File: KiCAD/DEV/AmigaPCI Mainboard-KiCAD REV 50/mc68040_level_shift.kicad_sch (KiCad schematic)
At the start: 28 parts, among them U801 74LVC1G17, U802 SN74LVC16T245DLR, U803 SN74LVC16T245DLR, U804 SN74LVC16T245DLR, U805 SN74LVC16T245DLR, U806 74LVC245, U807 74LVC245, U808 74LVC245, U809 74LVC245, U810 SN74LVC16T245DLR

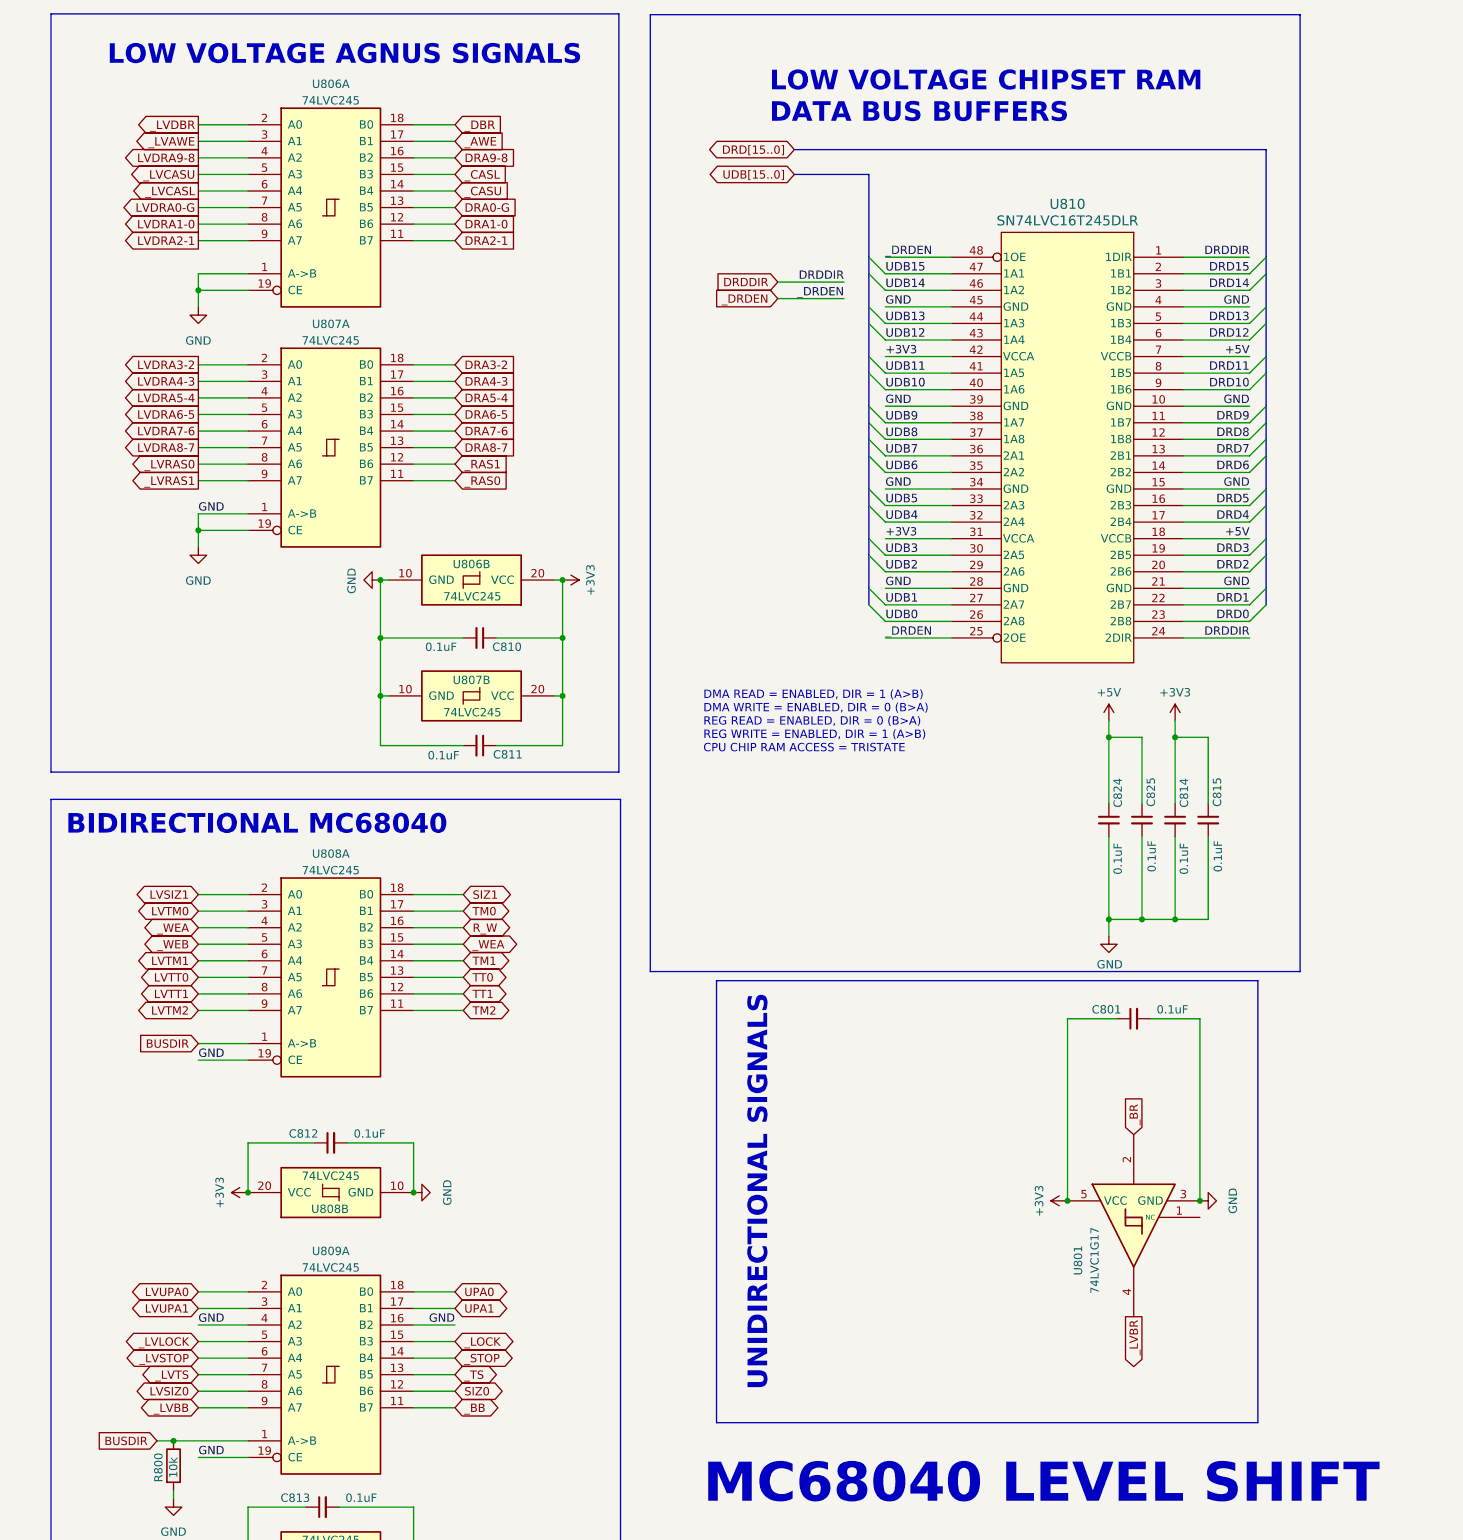
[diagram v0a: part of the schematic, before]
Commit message: More Rev 5.0 updates.
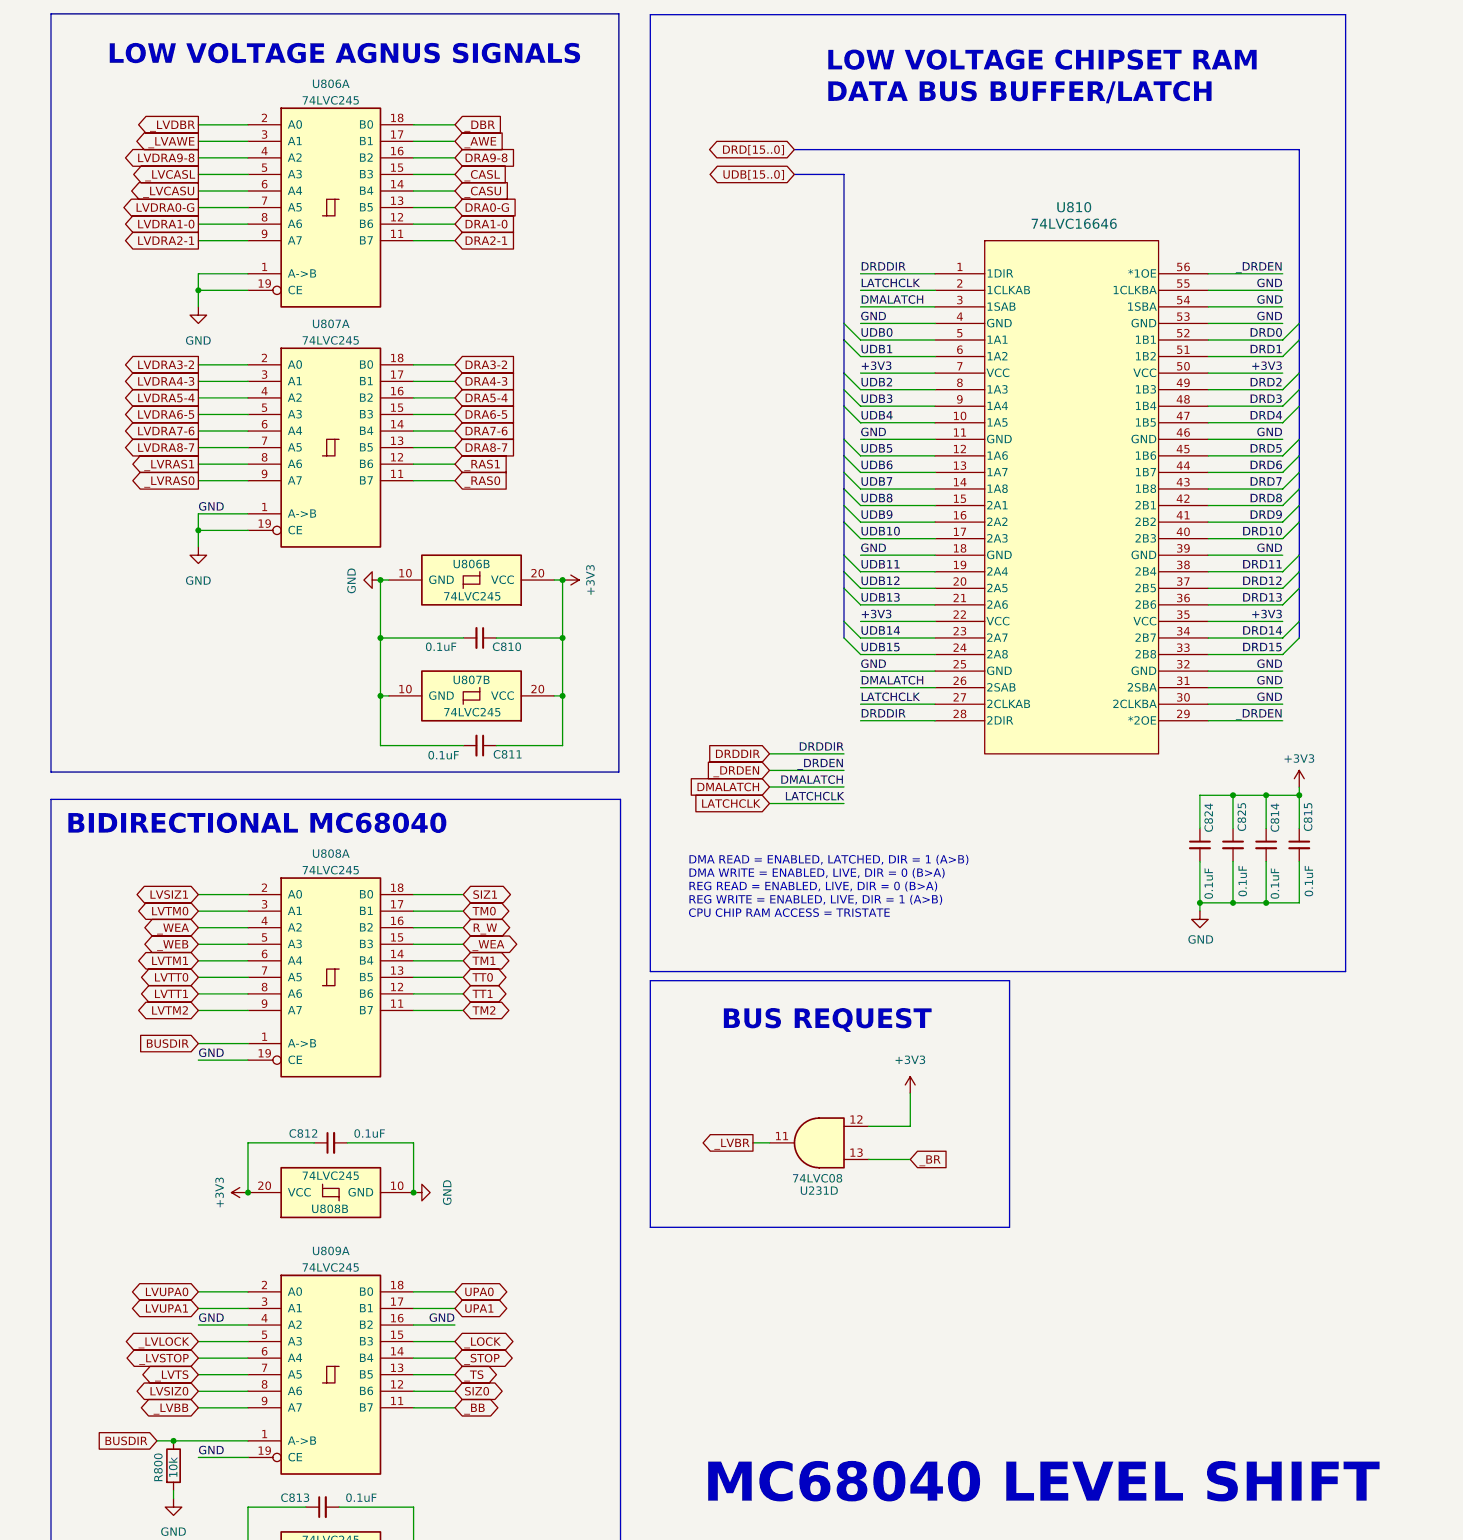
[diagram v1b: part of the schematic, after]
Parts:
- removed C801: 0.1uF, Capacitor_SMD:C_0603_1608Metric, symbol Device:C_Small
- removed U801: 74LVC1G17, Package_TO_SOT_SMD:SOT-23-5, symbol 74xGxx:74LVC1G17
- removed U810: SN74LVC16T245DLR, AmigaPCI:48-BSSOP, symbol AmigaPCI-Symbols:SN74LVC16T245DLR
- added U231: 74LVC08, Package_SO:TSSOP-14_4.4x5mm_P0.65mm, symbol 74xx:74LS08
- added U810: 74LVC16646, Package_SO:SSOP-56_7.5x18.5mm_P0.635mm, symbol AmigaPCI-Symbols:74LVC16646
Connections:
- net +3V3: now also C824.1, C825.1, U231.12, U810.22 (VCC), U810.35 (VCC), U810.50 (VCC), U810.7 (VCC)
- net +5V: no longer C824.1, C825.1
- net DRD0: now also U810.52 (1B1)
- net DRD1: now also U810.51 (1B2)
- net DRD10: now also U810.40 (2B3)
- net DRD11: now also U810.38 (2B4)
- net DRD12: now also U810.37 (2B5)
- net DRD13: now also U810.36 (2B6)
- net DRD14: now also U810.34 (2B7)
- net DRD15: now also U810.33 (2B8)
- net DRD2: now also U810.49 (1B3)
- net DRD3: now also U810.48 (1B4)
- net DRD4: now also U810.47 (1B5)
- net DRD5: now also U810.45 (1B6)
- net DRD6: now also U810.44 (1B7)
- net DRD7: now also U810.43 (1B8)
- net DRD8: now also U810.42 (2B1)
- net DRD9: now also U810.41 (2B2)
- net DRDDIR: now also U810.1 (1DIR), U810.28 (2DIR)
- net GND: now also U810.11 (GND), U810.18 (GND), U810.25 (GND), U810.30 (2CLKBA), U810.31 (2SBA), U810.32 (GND), U810.39 (GND), U810.4 (GND), U810.46 (GND), U810.53 (GND), U810.54 (1SBA), U810.55 (1CLKBA)
- net UDB0: now also U810.5 (1A1)
- net UDB1: now also U810.6 (1A2)
- net UDB10: now also U810.17 (2A3)
- net UDB11: now also U810.19 (2A4)
- net UDB12: now also U810.20 (2A5)
- net UDB13: now also U810.21 (2A6)
- net UDB14: now also U810.23 (2A7)
- net UDB15: now also U810.24 (2A8)
- net UDB2: now also U810.8 (1A3)
- net UDB3: now also U810.9 (1A4)
- net UDB4: now also U810.10 (1A5)
- net UDB5: now also U810.12 (1A6)
- net UDB6: now also U810.13 (1A7)
- net UDB7: now also U810.14 (1A8)
- net UDB8: now also U810.15 (2A1)
- net UDB9: now also U810.16 (2A2)
- net _BR: now also U231.13
- net _DRDEN: now also U810.29 (*2OE), U810.56 (*1OE)
- net _LVBR: now also U231.11
- net _LVCASL: now also U806.5 (A3); no longer U806.6 (A4)
- net _LVCASU: now also U806.6 (A4); no longer U806.5 (A3)
- net _LVRAS0: now also U807.9 (A7); no longer U807.8 (A6)
- net _LVRAS1: now also U807.8 (A6); no longer U807.9 (A7)
- new net DMALATCH: U810.26 (2SAB), U810.3 (1SAB)
- new net LATCHCLK: U810.2 (1CLKAB), U810.27 (2CLKAB)
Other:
- note added: "BUS REQUEST"
- note added: "DMA READ = ENABLED, LATCHED, DIR = 1 (A>B) DMA WRITE = ENABLED, LIVE, DIR = 0 (B>A) REG READ = ENABLED, LIVE, DIR = 0 (B>A) REG WRITE = ENABLED, LIVE, DIR = 1 (A>B) CPU CHIP RAM ACCESS = TRISTATE"
- note added: "LOW VOLTAGE CHIPSET RAM DATA BUS BUFFER/LATCH"
- note removed: "DMA READ = ENABLED, DIR = 1 (A>B) DMA WRITE = ENABLED, DIR = 0 (B>A) REG READ = ENABLED, DIR = 0 (B>A) REG WRITE = ENABLED, DIR = 1 (A>B) CPU CHIP RAM ACCESS = TRISTATE"
- note removed: "LOW VOLTAGE CHIPSET RAM DATA BUS BUFFERS"
- note removed: "UNIDIRECTIONAL SIGNALS"
- moved on the sheet: C814, C815, C824, C825
